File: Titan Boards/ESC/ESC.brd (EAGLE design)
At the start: 101.6 x 101.6 mm, 105 parts, among them IC2 74AHC1G08DBV, IC3 4002D, Q1 5.8A/30V/35mΩ, Q2 5.8A/30V/35mΩ, Q3 5.8A/30V/35mΩ, Q4 5.8A/30V/35mΩ, Q5 5.8A/30V/35mΩ, Q6 5.8A/30V/35mΩ, Q7 5.8A/30V/35mΩ, Q8 5.8A/30V/35mΩ

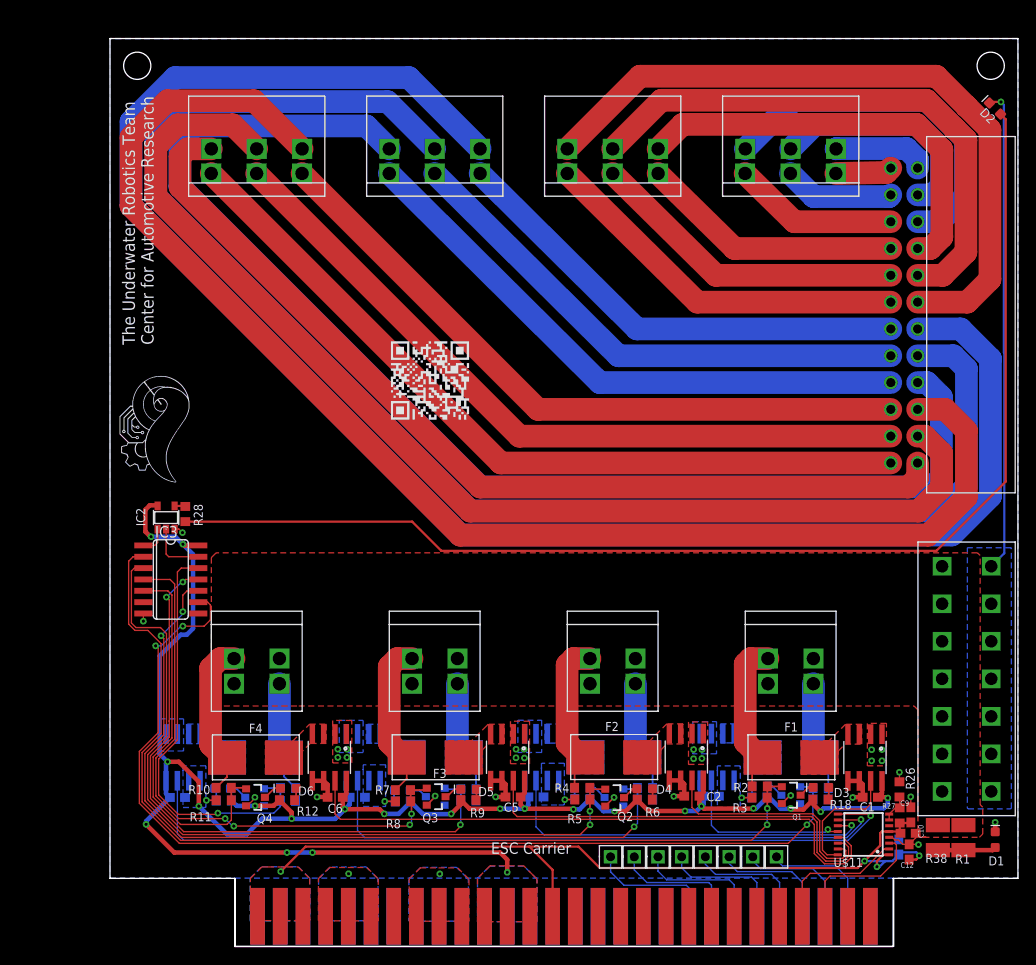
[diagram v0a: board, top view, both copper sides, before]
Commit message: ESC Updates + library additions
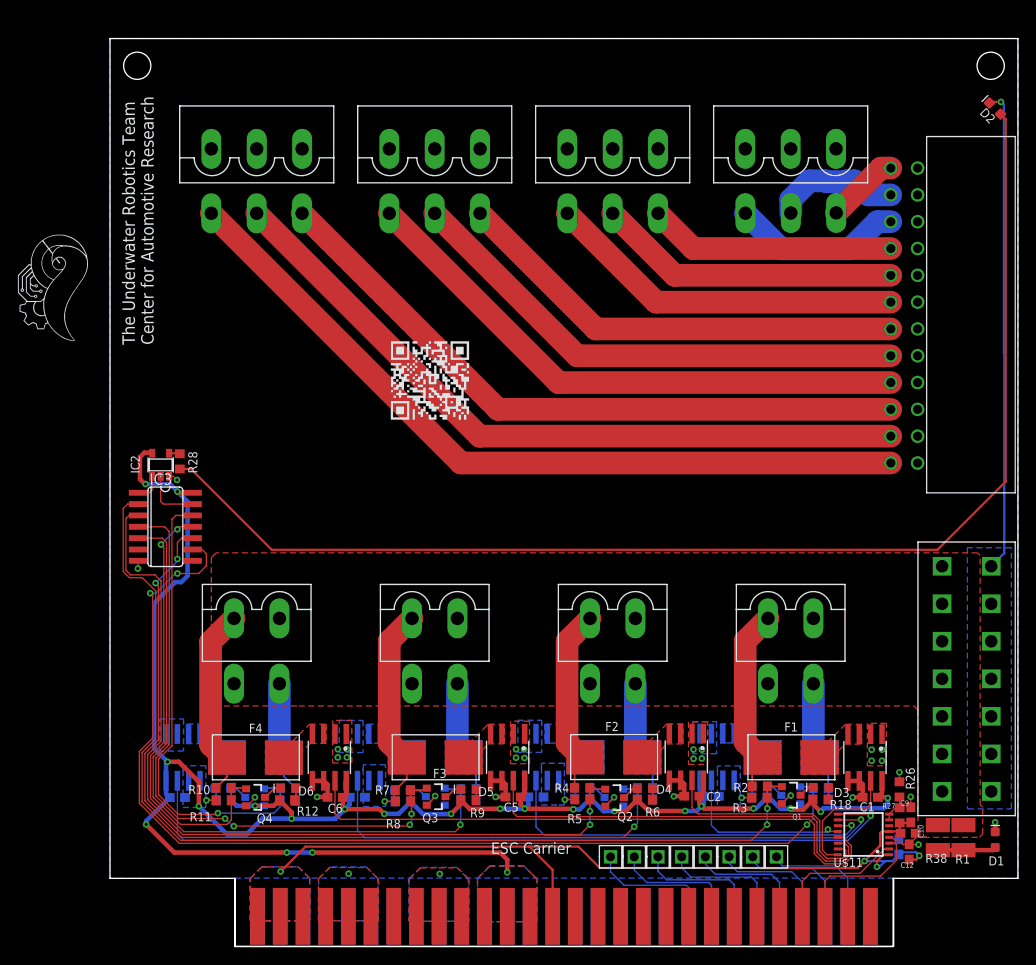
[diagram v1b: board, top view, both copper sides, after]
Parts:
- 2-PIN_1, 2-PIN_2, 2-PIN_3, 2-PIN_4, 2-PIN_5, 2-PIN_6, 2-PIN_7, 2-PIN_8: value 1711725 -> 1755736; device Screw_Terminals:1711725 -> Screw_Terminals:1755736
- 3-PIN_1, 3-PIN_2, 3-PIN_3, 3-PIN_4, 3-PIN_5, 3-PIN_6, 3-PIN_7, 3-PIN_8: value 1711738 -> 1755749; device Screw_Terminals:1711738 -> Screw_Terminals:1755749
- R12, R15, R18, R19, R22, R25, R6, R9: value 28 -> 150
- R28: value 15 -> 91
- moved IC2 5.92 mm to (5.67, 53.9)
- moved R28 5.92 mm to (7.82, 54.3)
- moved IC3 5.92 mm to (6.20, 47.0)
- moved 2-PIN_1 4.50 mm to (76.2, 36.7)
- moved 2-PIN_2 4.50 mm to (56.3, 36.7)
- moved 2-PIN_3 4.50 mm to (36.3, 36.7)
- moved 2-PIN_4 4.50 mm to (16.4, 36.7)
- moved 3-PIN_8 4.46 mm to (16.4, 82.0), turned to 180 degrees
- moved 3-PIN_6 4.46 mm to (56.3, 82.0), turned to 180 degrees
- moved 3-PIN_7 4.46 mm to (36.3, 82.0), turned to 180 degrees
- moved 3-PIN_5 4.43 mm to (76.2, 82.1), turned to 179.8 degrees
- turned 3-PIN_1 to 180 degrees
- turned 3-PIN_2 to 180 degrees
- turned 3-PIN_3 to 180 degrees
- turned 3-PIN_4 to 180 degrees
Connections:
- removed net N$1 (its old number): 24-PIN_CONNECTOR.1,BLUE, 3-PIN_4.BLUE
- removed net N$10: 24-PIN_CONNECTOR.7,BLUE, 3-PIN_1.BLUE
- removed net N$12: 24-PIN_CONNECTOR.7,WHITE, 3-PIN_1.WHITE
- removed net N$2 (its old number): 24-PIN_CONNECTOR.1,GREEN, 3-PIN_4.GREEN
- removed net N$3 (its old number): 24-PIN_CONNECTOR.1,WHITE, 3-PIN_4.WHITE
- removed net N$4 (its old number): 24-PIN_CONNECTOR.3,WHITE, 3-PIN_3.WHITE
- removed net N$7 (its old number): 24-PIN_CONNECTOR.5,BLUE, 3-PIN_2.BLUE
- removed net N$8 (its old number): 24-PIN_CONNECTOR.5,GREEN, 3-PIN_2.GREEN
- removed net N$9 (its old number): 24-PIN_CONNECTOR.5,WHITE, 3-PIN_2.WHITE
- net FUSE_1_TRIGGER: now also 2-PIN_1.P$1; no longer 2-PIN_1.BLACK
- net FUSE_2_TRIGGER: now also 2-PIN_2.P$1; no longer 2-PIN_2.BLACK
- net FUSE_3_TRIGGER: now also 2-PIN_3.P$1; no longer 2-PIN_3.BLACK
- net FUSE_4_TRIGGER: now also 2-PIN_4.P$1; no longer 2-PIN_4.BLACK
- net FUSE_5_TRIGGER: now also 2-PIN_5.P$1; no longer 2-PIN_5.BLACK
- net FUSE_6_TRIGGER: now also 2-PIN_6.P$1; no longer 2-PIN_6.BLACK
- net FUSE_7_TRIGGER: now also 2-PIN_7.P$1; no longer 2-PIN_7.BLACK
- net FUSE_8_TRIGGER: now also 2-PIN_8.P$1; no longer 2-PIN_8.BLACK
- net N$5: now also 24-PIN_CONNECTOR.7,BLUE, 3-PIN_1.WHITE; no longer 24-PIN_CONNECTOR.3,GREEN, 3-PIN_3.GREEN
- net N$6: now also 24-PIN_CONNECTOR.7,WHITE, 3-PIN_1.BLUE; no longer 24-PIN_CONNECTOR.3,BLUE, 3-PIN_3.BLUE
- net VOLTAGE_INPUT: now also 2-PIN_1.P$2, 2-PIN_2.P$2, 2-PIN_3.P$2, 2-PIN_4.P$2, 2-PIN_5.P$2, 2-PIN_6.P$2, 2-PIN_7.P$2, 2-PIN_8.P$2; no longer 2-PIN_1.RED, 2-PIN_2.RED, 2-PIN_3.RED, 2-PIN_4.RED, 2-PIN_5.RED, 2-PIN_6.RED, 2-PIN_7.RED, 2-PIN_8.RED
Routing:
- net N$4 (its old number): track 192.0 -> 0.00 mm
- net N$5: track 167.7 -> 0.00 mm
- net N$3 (its old number): track 155.1 -> 0.00 mm
- net N$6: track 142.2 -> 0.00 mm
- net N$2 (its old number): track 130.0 -> 0.00 mm
- net N$1 (its old number): track 105.8 -> 0.00 mm
- net N$7 (its old number): track 79.0 -> 0.00 mm
- net N$8 (its old number): track 62.7 -> 0.00 mm
- net N$9 (its old number): track 47.1 -> 0.00 mm
- net N$10: track 41.6 -> 0.00 mm
- net N$4: track 26.3 -> 0.00 mm
- net N$12: track 10.6 -> 0.00 mm
- net +5V: track 217.1 -> 223.2 mm
- net FAULT_5: track 112.4 -> 118.2 mm
- net FAULT_6: track 90.0 -> 95.6 mm
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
